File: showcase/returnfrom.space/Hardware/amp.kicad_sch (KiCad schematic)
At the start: 22 parts, among them U5 LM324

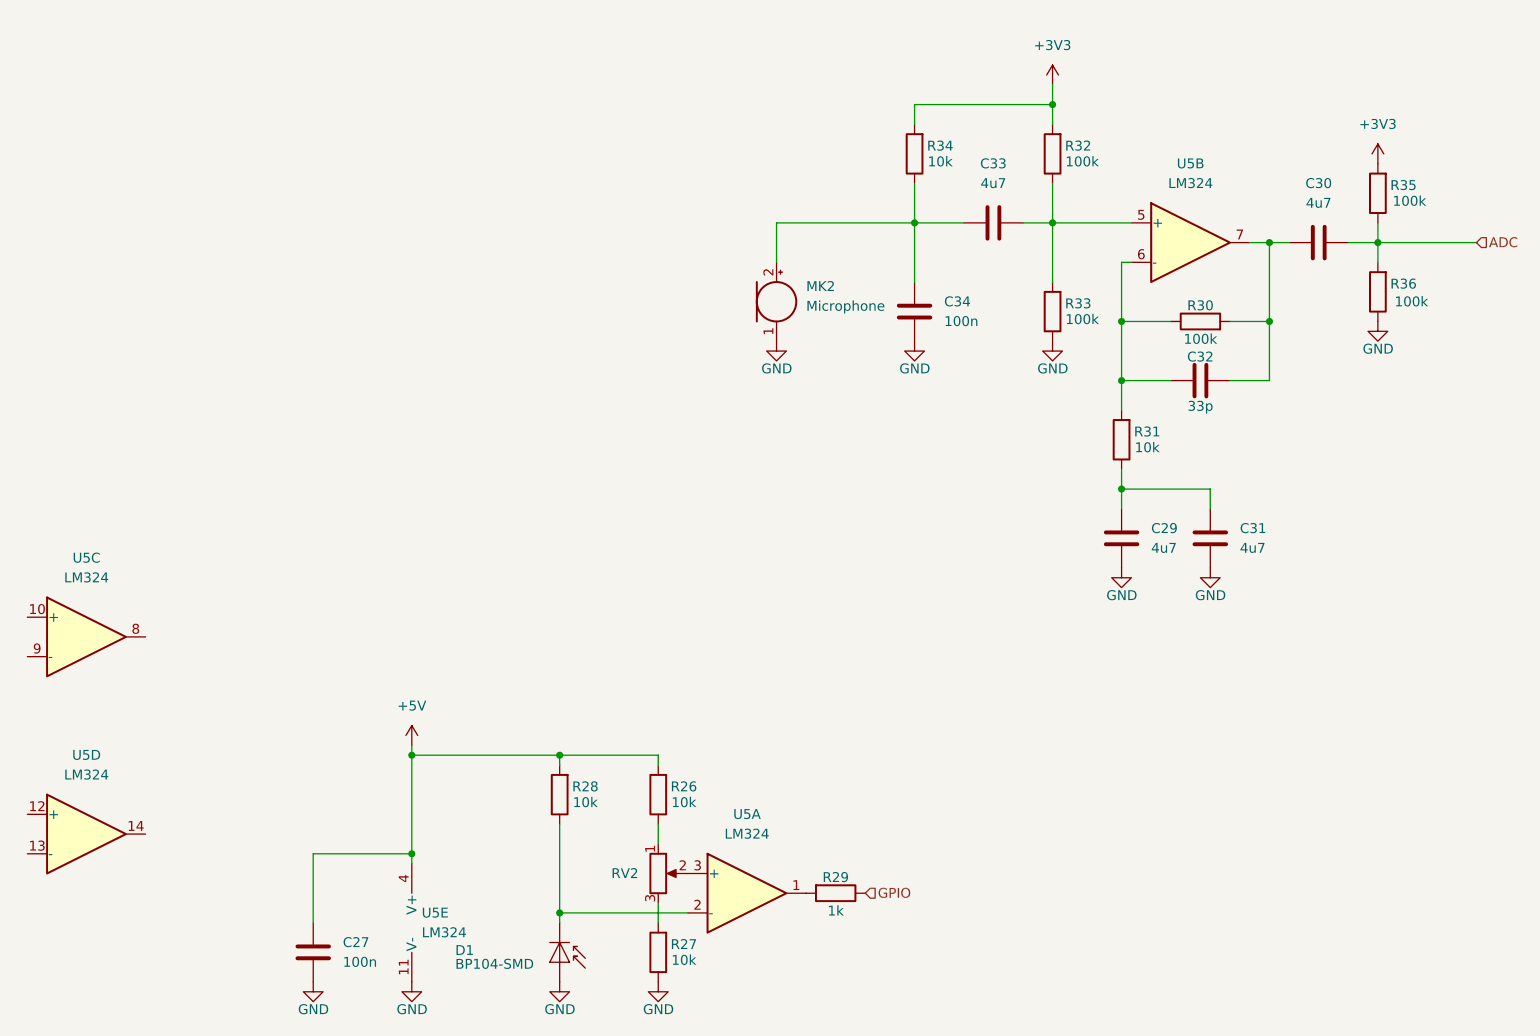
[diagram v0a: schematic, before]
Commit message: updated
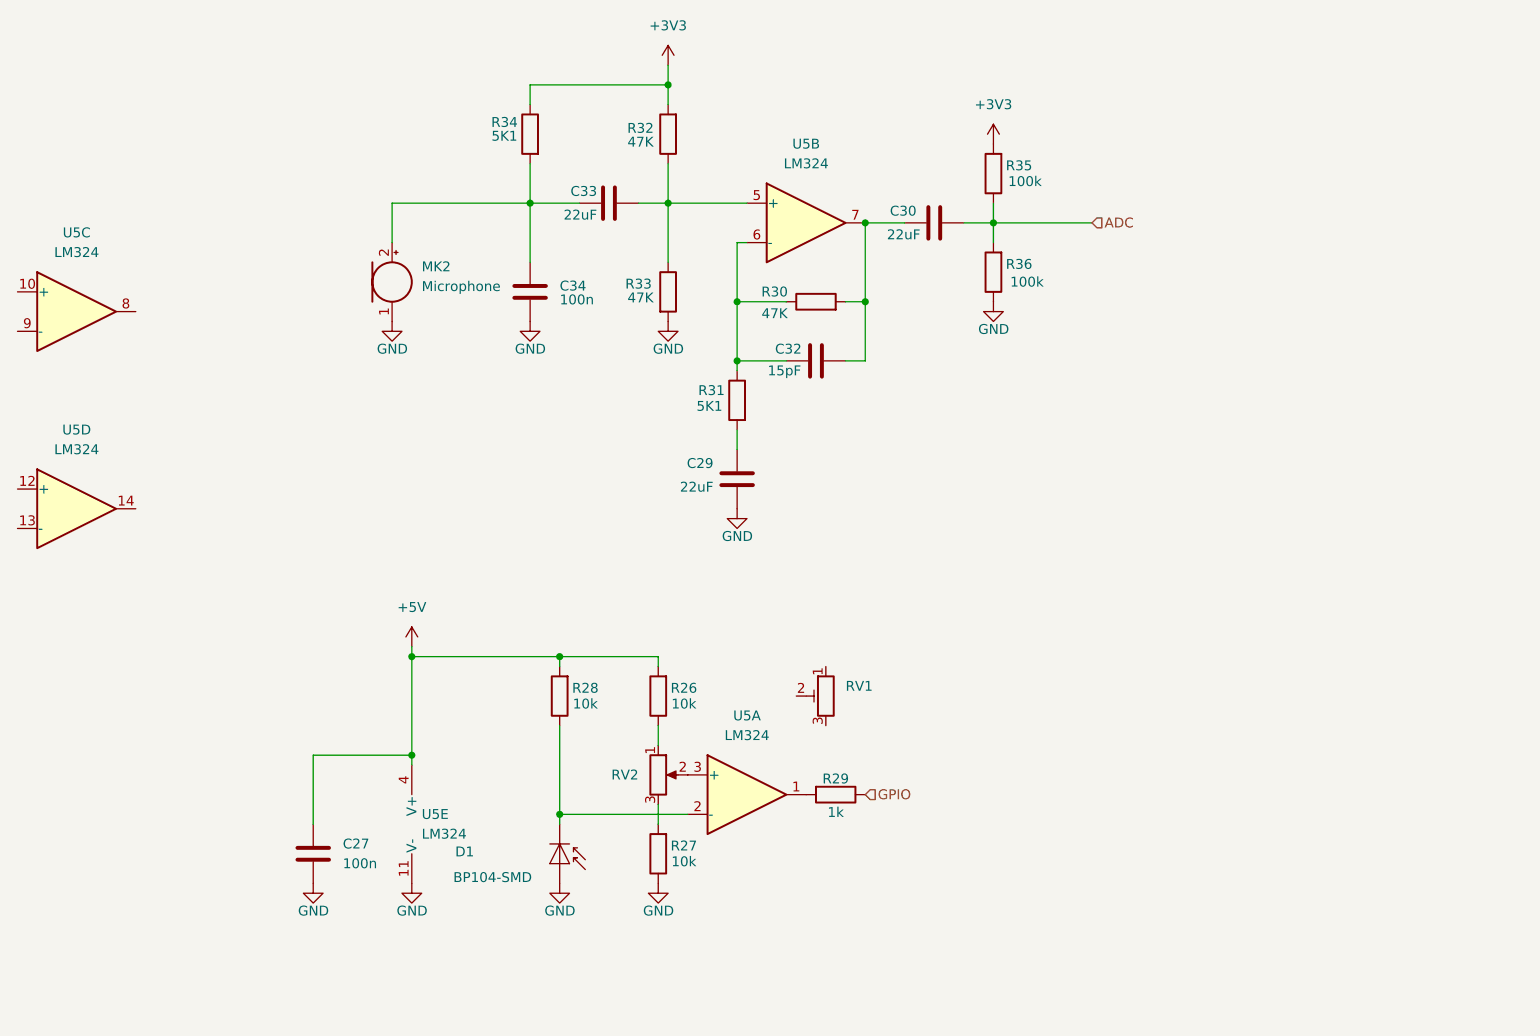
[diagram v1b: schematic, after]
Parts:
- removed C31: 4u7, Capacitor_SMD:C_0402_1005Metric, symbol Device:C
- added RV1: R_Potentiometer_Trim, Potentiometer_SMD:Potentiometer_Bourns_TC33X_Vertical, symbol Device:R_Potentiometer_Trim
- C29, C30, C33: value 4u7 -> 22uF; footprint Capacitor_SMD:C_0402_1005Metric -> Capacitor_SMD:C_0805_2012Metric
- C32: value 33p -> 15pF
- R30, R32, R33: value 100k -> 47K
- R31, R34: value 10k -> 5K1
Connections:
- net +3V3: now also R34.1; no longer R34.2
- net GND: now also R33.2; no longer R33.1
- net at C33.2, R32.1, U5.5 (+): now also R33.1; no longer R33.2
- net at C33.1, C34.1, MK2.2 (+): now also R34.2; no longer R34.1
- net at R31.1: now also C32.1, R30.1, U5.6 (-); no longer C29.1
- new net: C29.1, R31.2
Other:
- moved on the sheet: C27, C34, D1, MK2, R26, R27, R28, R29, R35, R36, RV2, U5A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
